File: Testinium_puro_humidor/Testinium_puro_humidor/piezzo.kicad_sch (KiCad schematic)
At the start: 1 part, among them J3 Piezzo

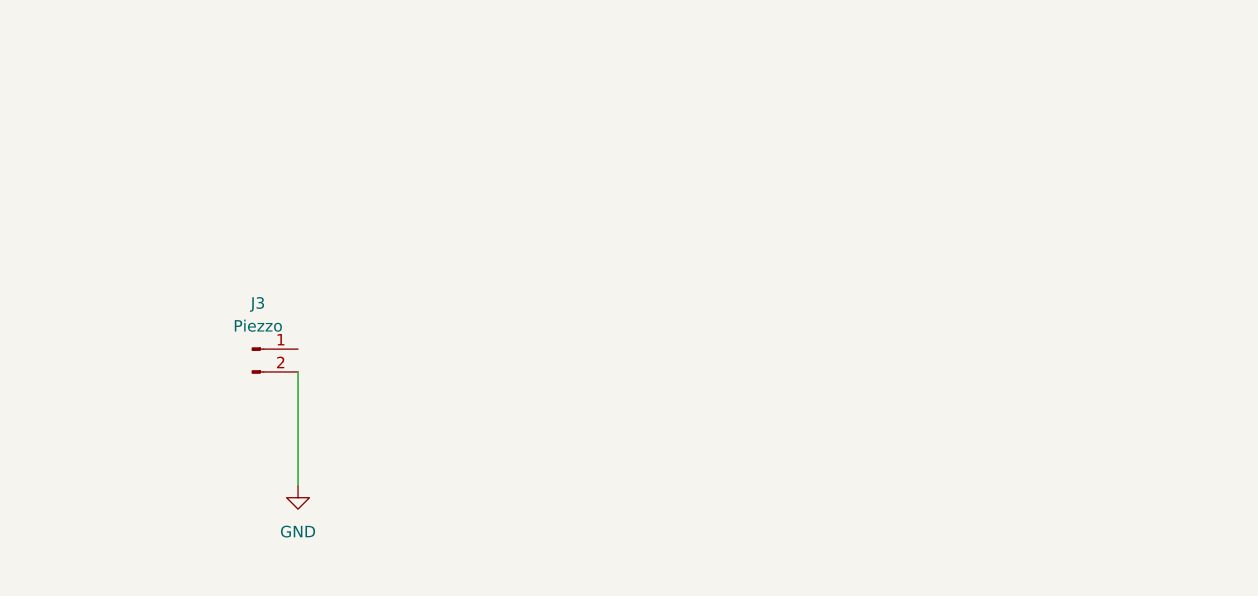
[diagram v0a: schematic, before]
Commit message: sematik tamamlandi
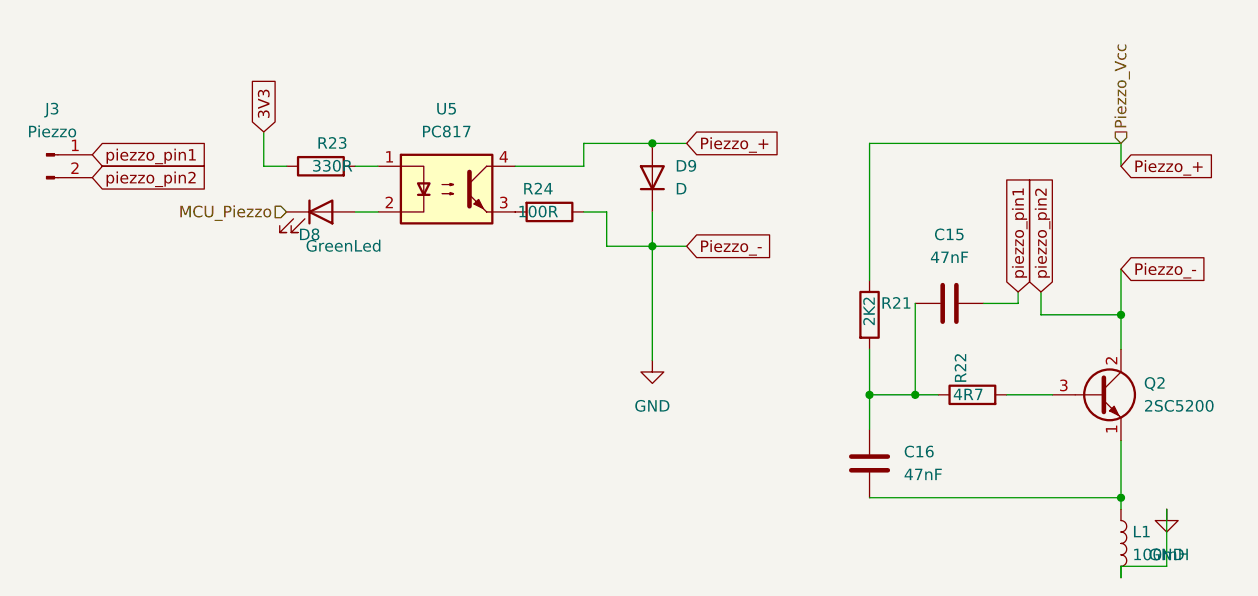
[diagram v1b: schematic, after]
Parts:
- added C15, C16: 47nF, Capacitor_SMD:C_0805_2012Metric, symbol Device:C
- added D8: GreenLed, LED_SMD:LED_0805_2012Metric, symbol Device:LED
- added D9: D, Diode_SMD:D_SMA, symbol Device:D
- added L1: 100mH, Inductor_SMD:L_10.4x10.4_H4.8, symbol Device:L
- added Q2: 2SC5200, Package_TO_SOT_THT:TO-92_Inline, symbol Transistor_BJT:2SC1815
- added R21: 2K2, Resistor_SMD:R_0805_2012Metric, symbol Device:R
- added R22: 4R7, Resistor_SMD:R_0805_2012Metric, symbol Device:R
- added R23: 330R, Resistor_SMD:R_0603_1608Metric, symbol Device:R
- added R24: 100R, Resistor_SMD:R_0603_1608Metric, symbol Device:R
- added U5: PC817, Package_SO:SOP-4_3.8x4.1mm_P2.54mm, symbol Isolator:PC817
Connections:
- net GND: now also D9.1 (K), L1.2, Q2.2 (C), R24.1
- net piezzo_pin1: now reaches J3.1 (Pin_1)
- net piezzo_pin1: now also C15.1
- new net: C16.1, L1.1, Q2.1 (E)
- new net: Q2.3 (B), R22.2
- new net: C15.2, C16.2, R21.2, R22.1
- new net: D8.2 (A), U5.2
- new net: R23.2, U5.1
- new net: R24.2, U5.3
- new net 3V3: R23.1
- new net MCU_Piezzo: D8.1 (K)
- new net Piezzo_+: D9.2 (A), R21.1, U5.4
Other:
- moved on the sheet: J3
